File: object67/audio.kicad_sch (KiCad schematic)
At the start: 56 parts, among them IC1 AK4493SEQ, IC2 TAA5242IRGER, IC3 LMK1C1104PWR, U1 RCJ-2223, Y3 ASDLJ-E-49.152MHZ-L-R-T, Y4 ASDLJ-E-45.1584MHz-L-R-T

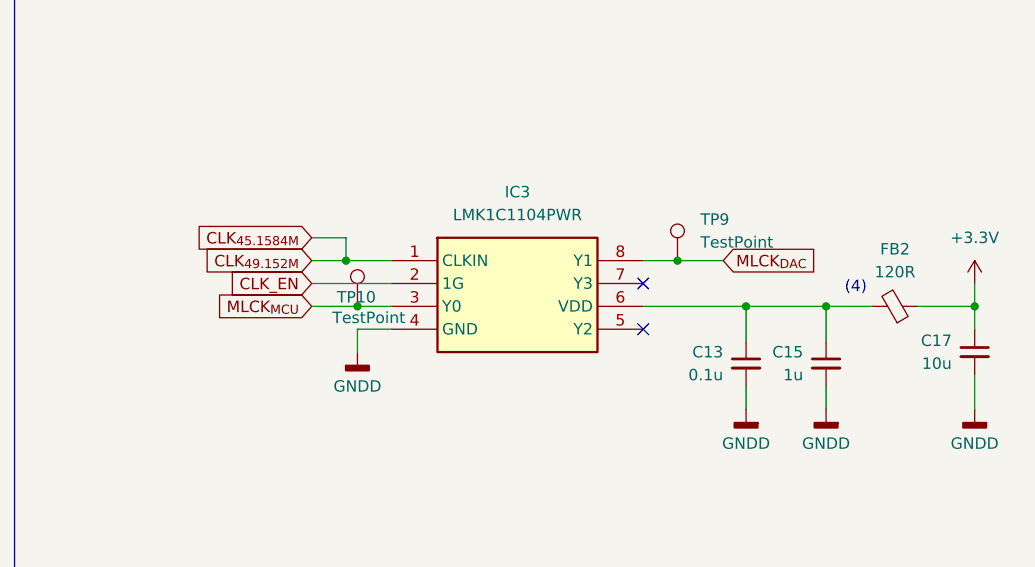
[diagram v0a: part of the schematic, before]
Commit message: More layouts
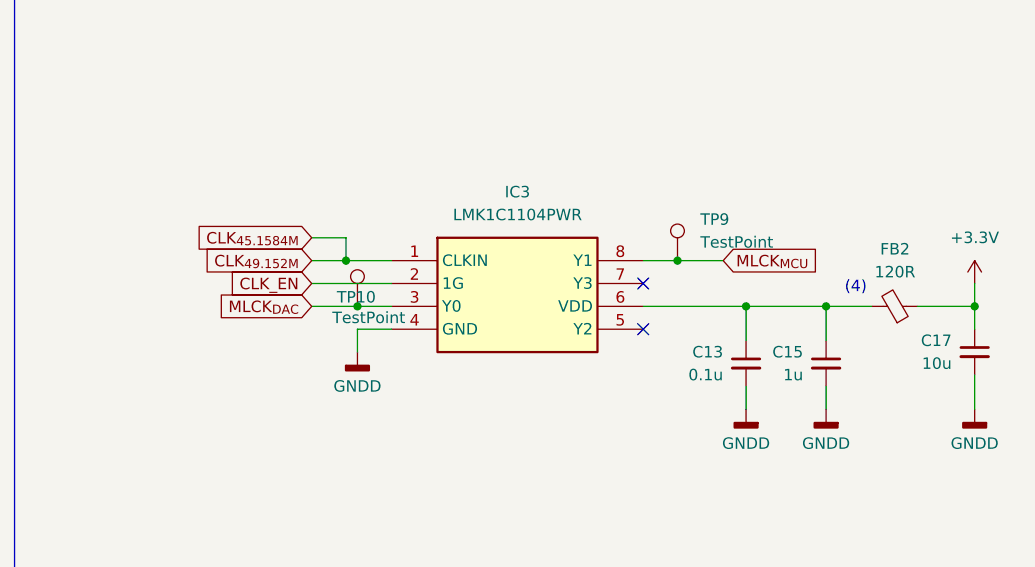
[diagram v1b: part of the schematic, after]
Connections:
- net MLCK_{DAC}: now also IC3.3 (Y0), TP10.1; no longer IC3.8 (Y1), TP9.1
- net MLCK_{MCU}: now also IC3.8 (Y1), TP9.1; no longer IC3.3 (Y0), TP10.1
